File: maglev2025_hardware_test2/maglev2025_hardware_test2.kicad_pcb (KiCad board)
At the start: 4 copper layers, 100 x 100 mm, 106 parts, among them J1 SWD, J2 PWRIn, U1 RY8411, U10 INA240A1PW, U11 INA240A1PW, U12 INA240A1PW, U2 TMAG5170-Q1, U3 STM32G474RBTx, U4 RS3236, U5 AT8236, U6 AT8236, U7 AT8236, U8 AT8236, U9 INA240A1PW, Y1 25MHz

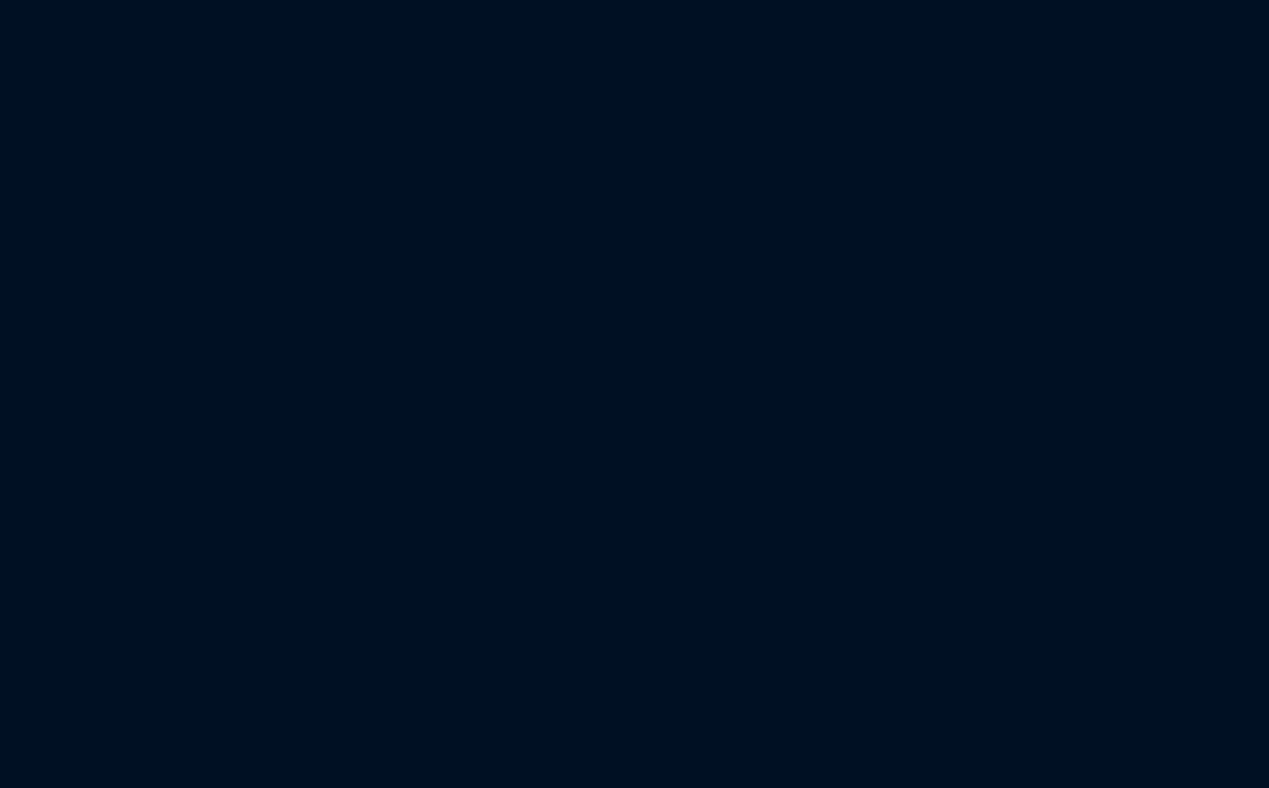
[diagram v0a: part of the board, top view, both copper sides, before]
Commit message: finish test2 sche
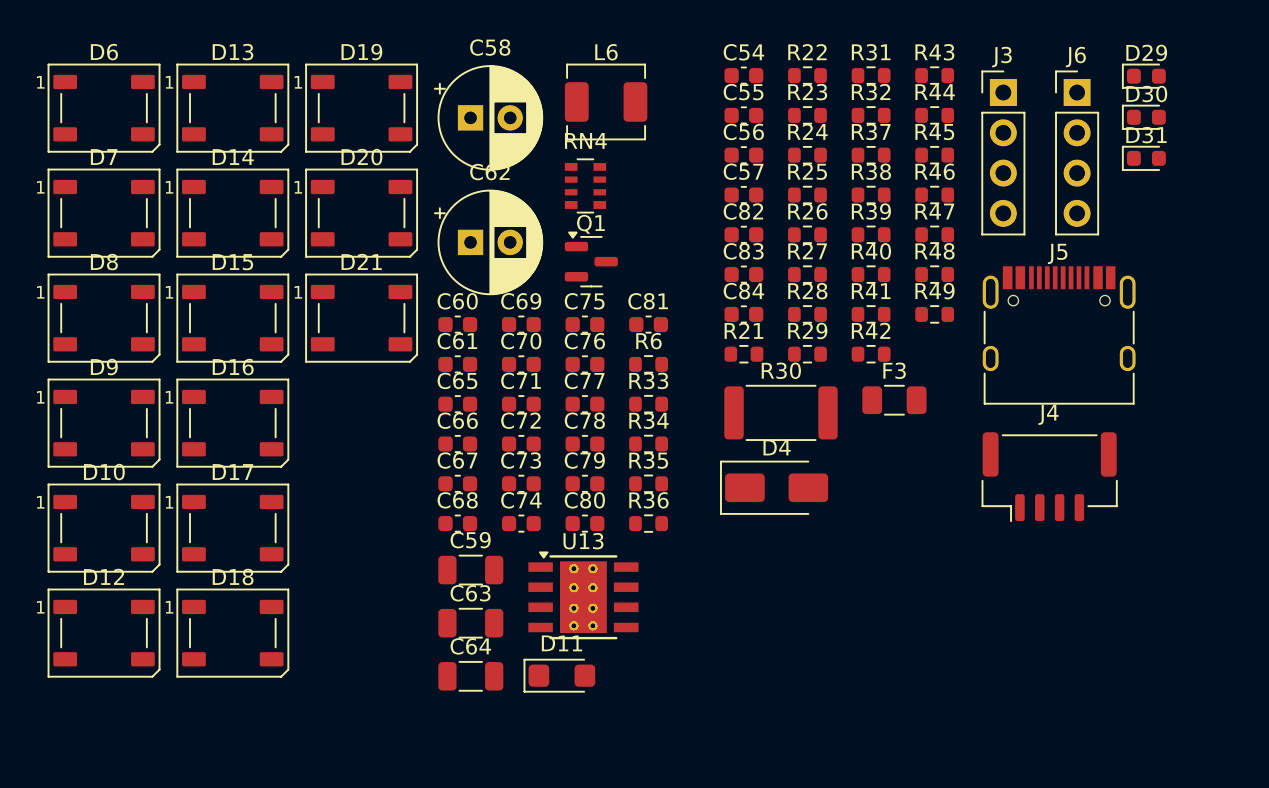
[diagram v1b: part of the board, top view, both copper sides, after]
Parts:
- added C54: 100n, Capacitor_SMD:C_0603_1608Metric, F.Cu at (-25.0, 69.7)
- added C55: 100n, Capacitor_SMD:C_0603_1608Metric, F.Cu at (-25.0, 72.2)
- added C56: 100n, Capacitor_SMD:C_0603_1608Metric, F.Cu at (-25.0, 74.7)
- added C57: 10n, Capacitor_SMD:C_0603_1608Metric, F.Cu at (-25.0, 77.2)
- added C58: 100u 16V, Capacitor_THT:CP_Radial_D6.3mm_P2.50mm, F.Cu at (-42.2, 72.3)
- added C59: 10u, Capacitor_SMD:C_1206_3216Metric, F.Cu at (-42.2, 100.8)
- added C60: 100n, Capacitor_SMD:C_0603_1608Metric, F.Cu at (-43.0, 85.4)
- added C61: 10n, Capacitor_SMD:C_0603_1608Metric, F.Cu at (-43.0, 87.9)
- added C62: 100u 16V, Capacitor_THT:CP_Radial_D6.3mm_P2.50mm, F.Cu at (-42.2, 80.2)
- added C63: 10u, Capacitor_SMD:C_1206_3216Metric, F.Cu at (-42.2, 104.2)
- added C64: 10u, Capacitor_SMD:C_1206_3216Metric, F.Cu at (-42.2, 107.5)
- added C65: 10u, Capacitor_SMD:C_0603_1608Metric, F.Cu at (-43.0, 90.4)
- added C66: 20p, Capacitor_SMD:C_0603_1608Metric, F.Cu at (-43.0, 92.9)
- added C67: 100n, Capacitor_SMD:C_0603_1608Metric, F.Cu at (-43.0, 95.4)
- added C68: 100n, Capacitor_SMD:C_0603_1608Metric, F.Cu at (-43.0, 97.9)
- added C69: 100n, Capacitor_SMD:C_0603_1608Metric, F.Cu at (-39.0, 85.4)
- added C70: 100n, Capacitor_SMD:C_0603_1608Metric, F.Cu at (-39.0, 87.9)
- added C71: 100n, Capacitor_SMD:C_0603_1608Metric, F.Cu at (-39.0, 90.4)
- added C72: 100n, Capacitor_SMD:C_0603_1608Metric, F.Cu at (-39.0, 92.9)
- added C73: 100n, Capacitor_SMD:C_0603_1608Metric, F.Cu at (-39.0, 95.4)
- added C74: 100n, Capacitor_SMD:C_0603_1608Metric, F.Cu at (-39.0, 97.9)
- added C75: 100n, Capacitor_SMD:C_0603_1608Metric, F.Cu at (-35.0, 85.4)
- added C76: 100n, Capacitor_SMD:C_0603_1608Metric, F.Cu at (-35.0, 87.9)
- added C77: 100n, Capacitor_SMD:C_0603_1608Metric, F.Cu at (-35.0, 90.4)
- added C78: 100n, Capacitor_SMD:C_0603_1608Metric, F.Cu at (-35.0, 92.9)
- added C79: 100n, Capacitor_SMD:C_0603_1608Metric, F.Cu at (-35.0, 95.4)
- added C80: 100n, Capacitor_SMD:C_0603_1608Metric, F.Cu at (-35.0, 97.9)
- added C81: 100n, Capacitor_SMD:C_0603_1608Metric, F.Cu at (-31.0, 85.4)
- added C82: 100n, Capacitor_SMD:C_0603_1608Metric, F.Cu at (-25.0, 79.7)
- added C83: 100n, Capacitor_SMD:C_0603_1608Metric, F.Cu at (-25.0, 82.2)
- added C84: 100n, Capacitor_SMD:C_0603_1608Metric, F.Cu at (-25.0, 84.7)
- added D10: WS2812B, LED_SMD:LED_WS2812B_PLCC4_5.0x5.0mm_P3.2mm, F.Cu at (-65.3, 98.2)
- added D11: DSS34, Diode_SMD:D_SMF, F.Cu at (-36.5, 107.5)
- added D12: WS2812B, LED_SMD:LED_WS2812B_PLCC4_5.0x5.0mm_P3.2mm, F.Cu at (-65.3, 104.8)
- added D13: WS2812B, LED_SMD:LED_WS2812B_PLCC4_5.0x5.0mm_P3.2mm, F.Cu at (-57.2, 71.7)
- added D14: WS2812B, LED_SMD:LED_WS2812B_PLCC4_5.0x5.0mm_P3.2mm, F.Cu at (-57.2, 78.3)
- added D15: WS2812B, LED_SMD:LED_WS2812B_PLCC4_5.0x5.0mm_P3.2mm, F.Cu at (-57.2, 85.0)
- added D16: WS2812B, LED_SMD:LED_WS2812B_PLCC4_5.0x5.0mm_P3.2mm, F.Cu at (-57.2, 91.6)
- added D17: WS2812B, LED_SMD:LED_WS2812B_PLCC4_5.0x5.0mm_P3.2mm, F.Cu at (-57.2, 98.2)
- added D18: WS2812B, LED_SMD:LED_WS2812B_PLCC4_5.0x5.0mm_P3.2mm, F.Cu at (-57.2, 104.8)
- added D19: WS2812B, LED_SMD:LED_WS2812B_PLCC4_5.0x5.0mm_P3.2mm, F.Cu at (-49.1, 71.7)
- added D20: WS2812B, LED_SMD:LED_WS2812B_PLCC4_5.0x5.0mm_P3.2mm, F.Cu at (-49.1, 78.3)
- added D21: WS2812B, LED_SMD:LED_WS2812B_PLCC4_5.0x5.0mm_P3.2mm, F.Cu at (-49.1, 85.0)
- added D29: LED, LED_SMD:LED_0603_1608Metric, F.Cu at (0.41, 69.7)
- added D30: LED, LED_SMD:LED_0603_1608Metric, F.Cu at (0.41, 72.3)
- added D31: LED, LED_SMD:LED_0603_1608Metric, F.Cu at (0.41, 74.9)
- added D4: DSS34, Diode_SMD:D_SMA, F.Cu at (-22.9, 95.7)
- added D6: WS2812B, LED_SMD:LED_WS2812B_PLCC4_5.0x5.0mm_P3.2mm, F.Cu at (-65.3, 71.7)
- added D7: WS2812B, LED_SMD:LED_WS2812B_PLCC4_5.0x5.0mm_P3.2mm, F.Cu at (-65.3, 78.3)
- added D8: WS2812B, LED_SMD:LED_WS2812B_PLCC4_5.0x5.0mm_P3.2mm, F.Cu at (-65.3, 85.0)
- added D9: WS2812B, LED_SMD:LED_WS2812B_PLCC4_5.0x5.0mm_P3.2mm, F.Cu at (-65.3, 91.6)
- added F3: 5A, Fuse:Fuse_1206_3216Metric, F.Cu at (-15.5, 90.1)
- added J3: Conn_01x04, Connector_PinHeader_2.54mm:PinHeader_1x04_P2.54mm_Vertical, F.Cu at (-8.62, 70.7)
- added J4: Conn_01x04_MountingPin, Connector_JST:JST_GH_BM04B-GHS-TBT_1x04-1MP_P1.25mm_Vertical, F.Cu at (-5.70, 95.0)
- added J5: USB_C_Receptacle_USB2.0, Connector_USB:USB_C_Receptacle_HRO_TYPE-C-31-M-12, F.Cu at (-5.09, 86.5)
- added J6: Conn_01x04, Connector_PinHeader_2.54mm:PinHeader_1x04_P2.54mm_Vertical, F.Cu at (-3.96, 70.7)
- added L6: 15u, Inductor_SMD:L_Sunlord_MWSA0402S, F.Cu at (-33.7, 71.3)
- added Q1: AO3400A, Package_TO_SOT_SMD:SOT-23, F.Cu at (-34.6, 81.4)
- added R21: 33r, Resistor_SMD:R_0603_1608Metric, F.Cu at (-25.0, 87.2)
- added R22: 33r, Resistor_SMD:R_0603_1608Metric, F.Cu at (-21.0, 69.7)
- added R23: 4.7k, Resistor_SMD:R_0603_1608Metric, F.Cu at (-21.0, 72.2)
- added R24: 4.7k, Resistor_SMD:R_0603_1608Metric, F.Cu at (-21.0, 74.7)
- added R25: 33r, Resistor_SMD:R_0603_1608Metric, F.Cu at (-21.0, 77.2)
- added R26: 33r, Resistor_SMD:R_0603_1608Metric, F.Cu at (-21.0, 79.7)
- added R27: 1M, Resistor_SMD:R_0603_1608Metric, F.Cu at (-21.0, 82.2)
- added R28: 33r, Resistor_SMD:R_0603_1608Metric, F.Cu at (-21.0, 84.7)
- added R29: 33r, Resistor_SMD:R_0603_1608Metric, F.Cu at (-21.0, 87.2)
- added R30: R_US, Resistor_SMD:R_2512_6332Metric, F.Cu at (-22.6, 90.9)
- added R31: 10k, Resistor_SMD:R_0603_1608Metric, F.Cu at (-17.0, 69.7)
- added R32: 1k, Resistor_SMD:R_0603_1608Metric, F.Cu at (-17.0, 72.2)
- added R33: 3.24k, Resistor_SMD:R_0603_1608Metric, F.Cu at (-31.0, 90.4)
- added R34: 10k, Resistor_SMD:R_0603_1608Metric, F.Cu at (-31.0, 92.9)
- added R35: 33r, Resistor_SMD:R_0603_1608Metric, F.Cu at (-31.0, 95.4)
- added R36: 33R, Resistor_SMD:R_0603_1608Metric, F.Cu at (-31.0, 97.9)
- added R37: 33r, Resistor_SMD:R_0603_1608Metric, F.Cu at (-17.0, 74.7)
- added R38: 33r, Resistor_SMD:R_0603_1608Metric, F.Cu at (-17.0, 77.2)
- added R39: 33r, Resistor_SMD:R_0603_1608Metric, F.Cu at (-17.0, 79.7)
- added R40: 33r, Resistor_SMD:R_0603_1608Metric, F.Cu at (-17.0, 82.2)
- added R41: 330, Resistor_SMD:R_0603_1608Metric, F.Cu at (-17.0, 84.7)
- added R42: 1k, Resistor_SMD:R_0603_1608Metric, F.Cu at (-17.0, 87.2)
- added R43: 10k, Resistor_SMD:R_0603_1608Metric, F.Cu at (-12.9, 69.7)
- added R44: 330, Resistor_SMD:R_0603_1608Metric, F.Cu at (-12.9, 72.2)
- added R45: 1k, Resistor_SMD:R_0603_1608Metric, F.Cu at (-12.9, 74.7)
- added R46: 10k, Resistor_SMD:R_0603_1608Metric, F.Cu at (-12.9, 77.2)
- added R47: 330, Resistor_SMD:R_0603_1608Metric, F.Cu at (-12.9, 79.7)
- added R48: 1k, Resistor_SMD:R_0603_1608Metric, F.Cu at (-12.9, 82.2)
- added R49: 10k, Resistor_SMD:R_0603_1608Metric, F.Cu at (-12.9, 84.7)
- added R6: 10k, Resistor_SMD:R_0603_1608Metric, F.Cu at (-31.0, 87.9)
- added RN4: 33x4, Resistor_SMD:R_Array_Convex_4x0603, F.Cu at (-35.0, 76.6)
- added U13: TPS5430DDA, Package_SO:TI_SO-PowerPAD-8_ThermalVias, F.Cu at (-35.1, 102.6)
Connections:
- C1 pad 1: VREF -> VREF_MCU
- C2 pad 1: VREF -> VREF_MCU
- R11 pad 1: GND -> GND_PWR
- R12 pad 1: GND -> GND_PWR
- R13 pad 1: GND -> GND_PWR
- R14 pad 1: GND -> GND_PWR
- R20 pad 1: Net-(U3-PA15) -> Net-(U3-PA13)
- R4 pad 1: Net-(U3-PB7) -> Net-(U3-PA3)
- U3 pad 10: unconnected-(U3-PC2-Pad10) -> ISENSE_D_MCU
- U3 pad 11: unconnected-(U3-PC3-Pad11) -> ISENSE_C_MCU
- U3 pad 12: unconnected-(U3-PA0-Pad12) -> ISENSE_B_MCU
- U3 pad 13: unconnected-(U3-PA1-Pad13) -> ISENSE_A_MCU
- U3 pad 17: unconnected-(U3-PA3-Pad17) -> Net-(U3-PA3)
- U3 pad 18: ISENSE_A_MCU -> Net-(RN4-R4.1)
- U3 pad 19: unconnected-(U3-PA5-Pad19) -> Net-(RN4-R3.1)
- U3 pad 2: unconnected-(U3-PC13-Pad2) -> /PC13
- U3 pad 20: ISENSE_B_MCU -> Net-(RN4-R2.1)
- U3 pad 21: unconnected-(U3-PA7-Pad21) -> Net-(RN4-R1.1)
- U3 pad 22: ISENSE_C_MCU -> /USART1_TX
- U3 pad 23: unconnected-(U3-PC5-Pad23) -> /USART1_RX
- U3 pad 24: unconnected-(U3-PB0-Pad24) -> VREF_MCU
- U3 pad 25: unconnected-(U3-PB1-Pad25) -> VREF
- U3 pad 26: ISENSE_D_MCU -> unconnected-(U3-PB2-Pad26)
- U3 pad 28: VREF -> VREF_MCU
- U3 pad 3: unconnected-(U3-PC14-Pad3) -> /PC14
- U3 pad 33: unconnected-(U3-PB11-Pad33) -> /OPAMP4_VINP
- U3 pad 4: unconnected-(U3-PC15-Pad4) -> /PC15
- U3 pad 40: unconnected-(U3-PC8-Pad40) -> I2C3_SCL
- U3 pad 41: unconnected-(U3-PC9-Pad41) -> I2C3_SDA
- U3 pad 49: unconnected-(U3-PA13-Pad49) -> Net-(U3-PA13)
- U3 pad 51: Net-(U3-PA15) -> unconnected-(U3-PA15-Pad51)
- U3 pad 52: unconnected-(U3-PC10-Pad52) -> /PC10
- U3 pad 53: unconnected-(U3-PC11-Pad53) -> /PC11
- U3 pad 54: unconnected-(U3-PC12-Pad54) -> /PC12
- U3 pad 55: unconnected-(U3-PD2-Pad55) -> /PD2
- U3 pad 56: Net-(RN2-R4.1) -> /PB3
- U3 pad 57: Net-(RN2-R3.1) -> /UCPD1_CC2
- U3 pad 58: Net-(RN2-R2.1) -> unconnected-(U3-PB5-Pad58)
- U3 pad 59: Net-(RN2-R1.1) -> /UCPD1_CC1
- U3 pad 60: Net-(U3-PB7) -> unconnected-(U3-PB7-Pad60)
- U3 pad 62: Net-(U3-PB9) -> unconnected-(U3-PB9-Pad62)
- U3 pad 8: unconnected-(U3-PC0-Pad8) -> BUZZER
- U3 pad 9: unconnected-(U3-PC1-Pad9) -> VSENSE_VBUS
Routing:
- net (no net): track 0.00 -> 40.3 mm, vias 0 -> 2
- net Net-(U3-PA15): track 34.8 -> 0.00 mm, vias 2 -> 0
- net Net-(U3-PB7): track 5.46 -> 0.00 mm
